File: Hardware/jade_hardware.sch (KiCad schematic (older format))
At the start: 37 parts, among them J1 PJ302M, J2 PJ302M, J3 PJ302M, J4 PJ302M, J5 Conn_02x05_Odd_Even, J6 Conn_02x03_Odd_Even, J7 PJ302M, J8 PJ302M, Q1 MMBT3904, Q2 MMBT3904, Q3 MMBT3904, Q4 MMBT3904, U1 SeeeduinoXIAO, U2 LM358

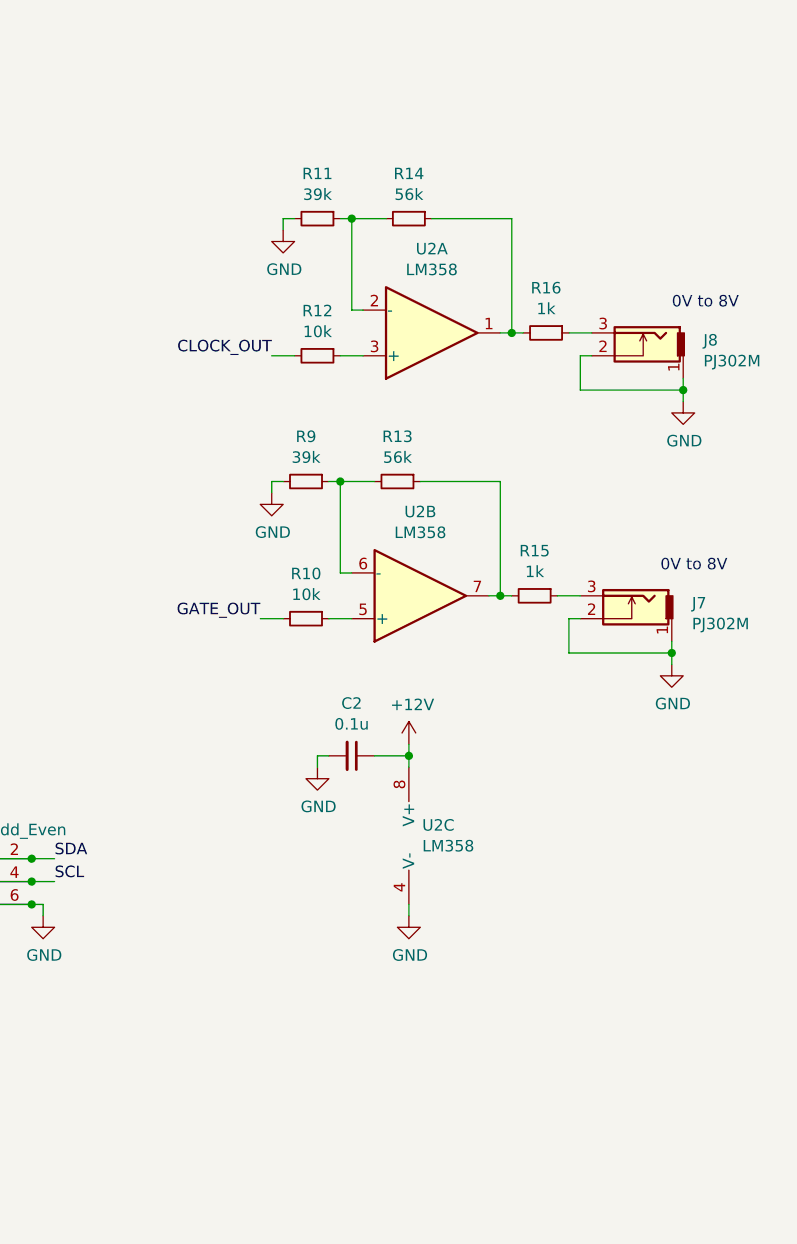
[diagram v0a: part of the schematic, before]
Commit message: Eurorack main board Rev.B
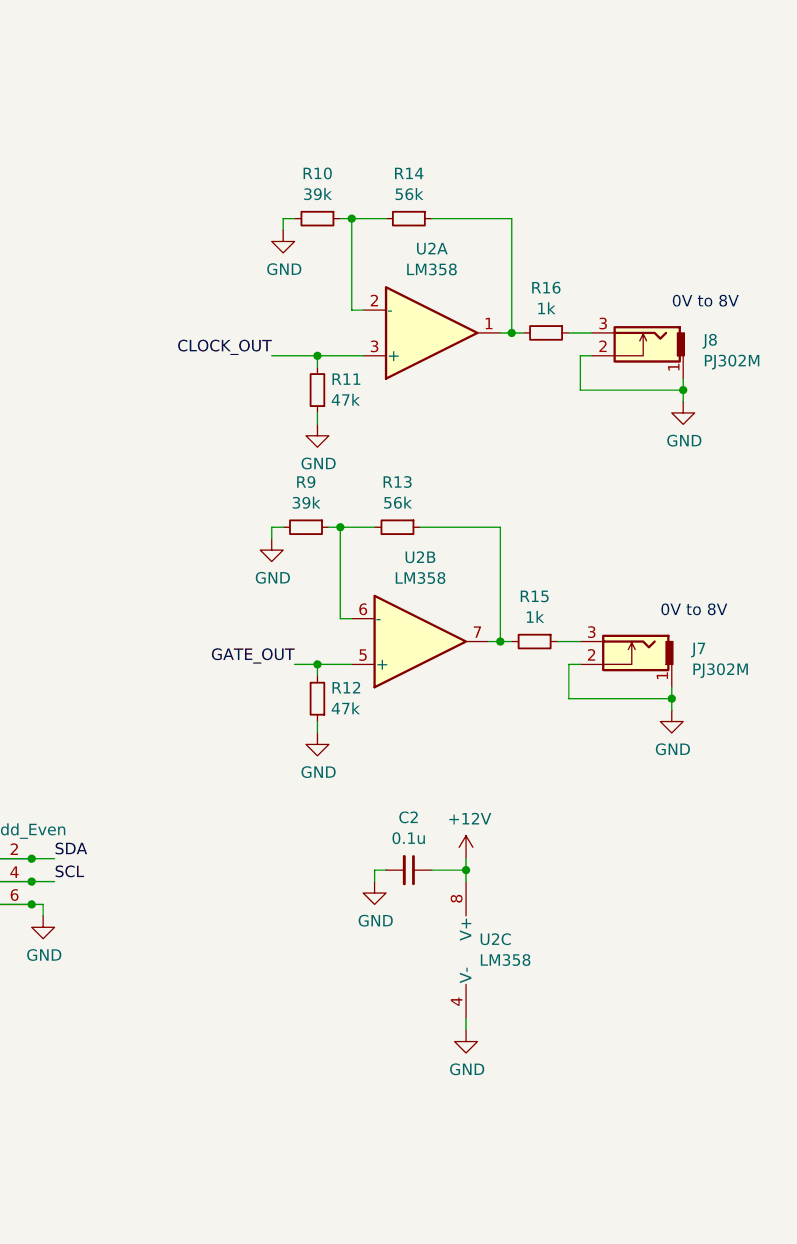
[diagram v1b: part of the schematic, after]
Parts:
- removed R10: 10k, Resistor_SMD:R_0603_1608Metric_Pad0.98x0.95mm_HandSolder, symbol Device:R_Small
- added R11: 47k, Resistor_SMD:R_0603_1608Metric_Pad0.98x0.95mm_HandSolder, symbol Device:R_Small
- R12: value 10k -> 47k
- renumbered R11 to R10
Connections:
- net CLOCK_OUT: now also U2.3 (+), R11.2; no longer R12.2
- net GATE_OUT: now also R12.2, U2.5 (+)
- net GND: now also R12.1, R11.1
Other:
- moved on the sheet: C2, J7, R13, R15, R9, U2B, U2C
